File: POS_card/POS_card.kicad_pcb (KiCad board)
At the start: 2 copper layers, 74 parts, among them J1 molex3.0 2x2, J2 UART, J3 SWD, J4 USB_B_Micro, J5 Conn_01x02, J6 Encoder1, J7 Encoder2, Q1 BSS138, Q2 BSS138, Q3 BSS138, Q4 BSS138, Q5 BSS138, Q6 BSS138, SW1 SW_Push, SW2 SW_Push, U1 RP2040, U2 MCP2517FD-xSL, U3 MCP2562-E-SN, U4 NCP1117-3.3_SOT223, U5 W25Q128JVS, Y1 ASEAIG-40MHZ-C-S-T, Y2 ABLS-12.000MHZ-B4-T

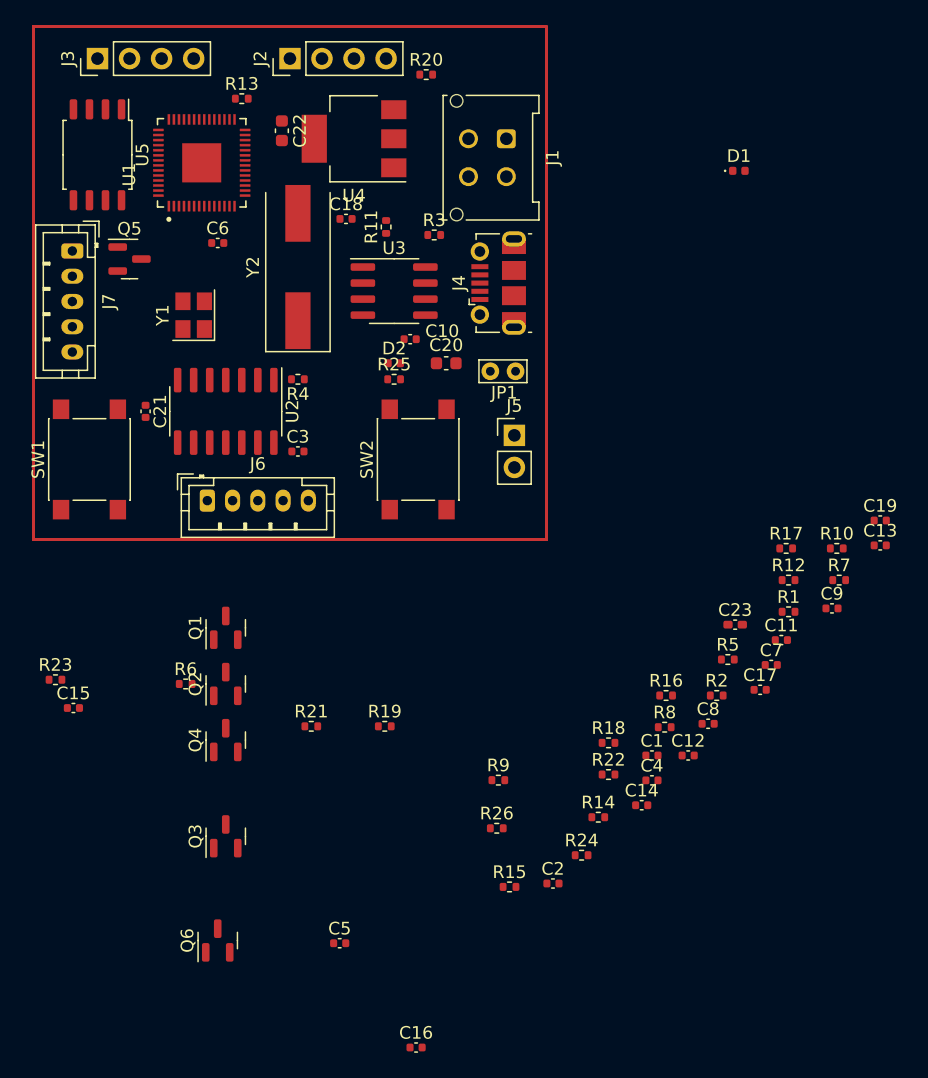
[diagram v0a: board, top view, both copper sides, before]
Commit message: new shield
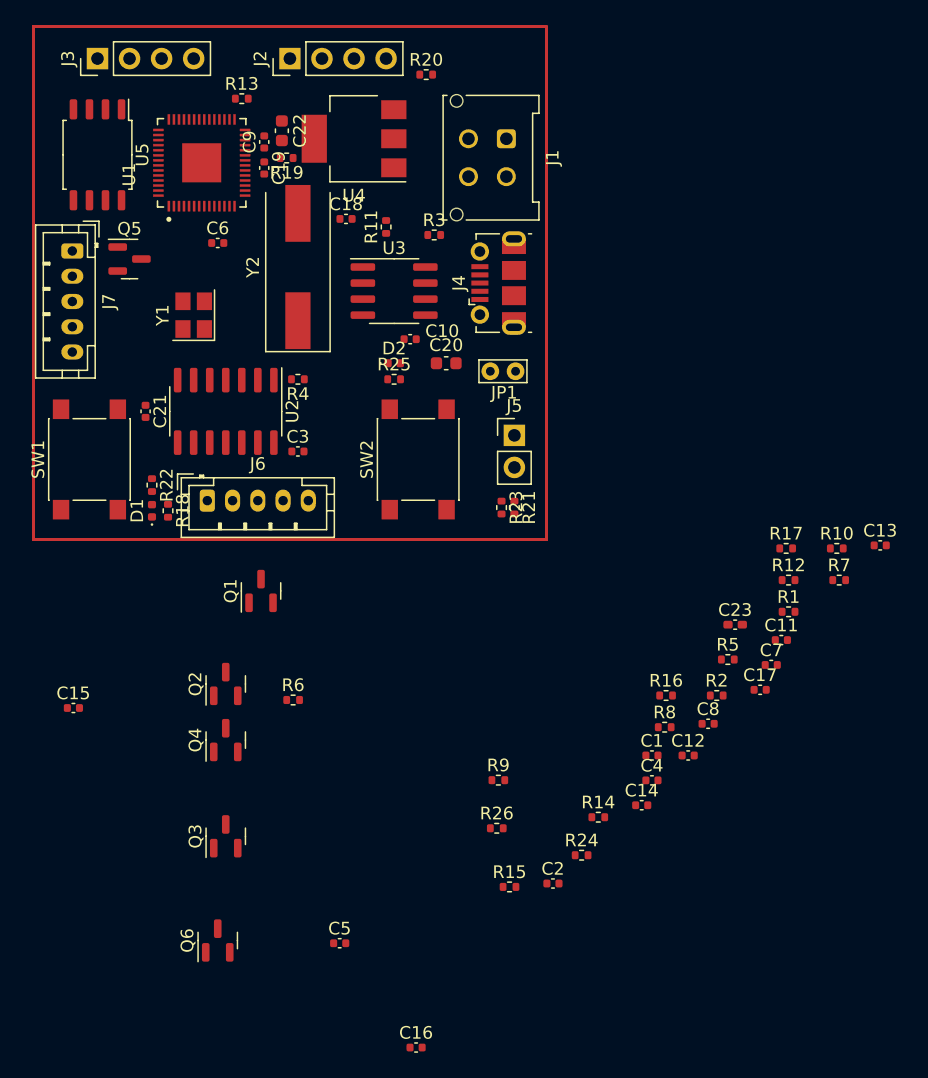
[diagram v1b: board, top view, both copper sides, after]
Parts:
- moved C9 58.2 mm to (94.5, 85.3), turned to 90 degrees
- moved C19 56.2 mm to (94.5, 87.4), turned to -90 degrees
- moved D1 53.7 mm to (85.6, 114.6), turned to 90 degrees
- moved R19 45.7 mm to (96.3, 86.6), turned to 180 degrees
- moved R22 42.8 mm to (85.6, 112.5), turned to -90 degrees
- moved R18 39.4 mm to (86.9, 114.6), turned to -90 degrees
- moved R23 37.9 mm to (113.3, 114.3), turned to -90 degrees
- moved R21 23.6 mm to (114.3, 114.3), turned to -90 degrees
- moved R6 8.61 mm to (96.8, 129.5)
- moved Q1 4.04 mm to (94.2, 120.9)
